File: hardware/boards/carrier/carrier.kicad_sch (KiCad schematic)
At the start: 4 parts, among them J1 XT30PW(2+2)-M.G.B_SLOT, J2 DC+_OUT, J3 DC-_OUT, J4 I2C_OUT

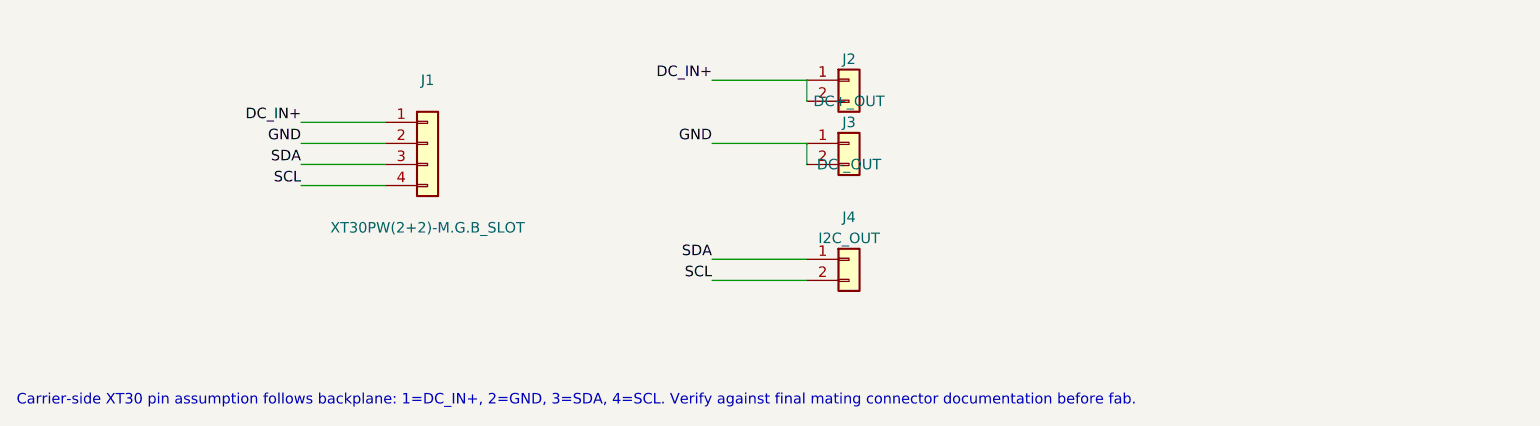
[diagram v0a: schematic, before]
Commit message: chore: checkpoint current project updates
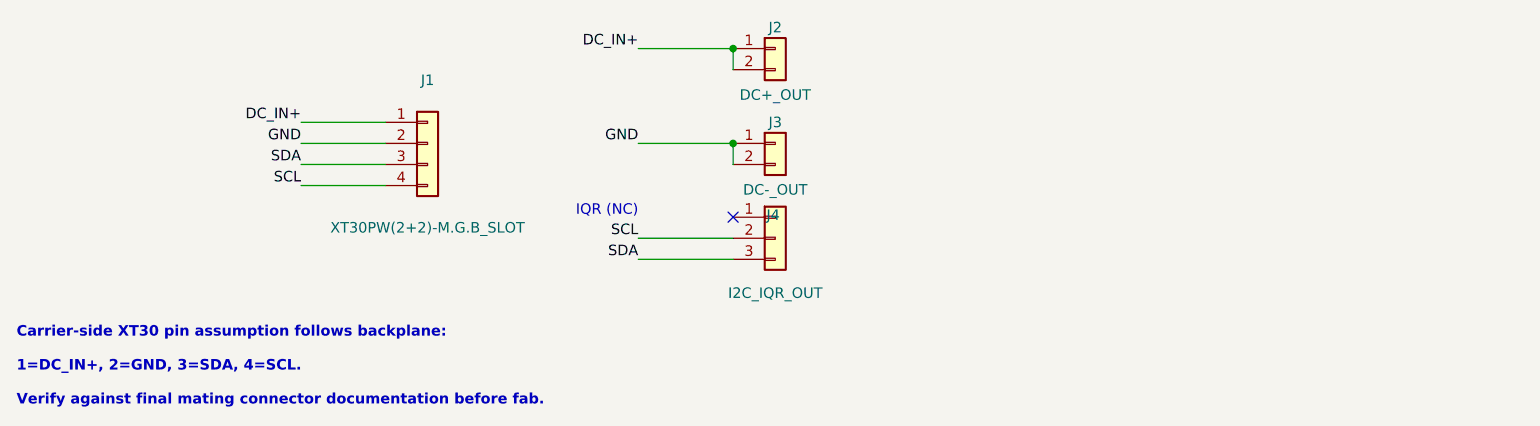
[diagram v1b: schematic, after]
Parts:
- J4: value I2C_OUT -> I2C_IQR_OUT; footprint Connector_PinHeader_2.54mm:PinHeader_1x02_P2.54mm_Vertical -> Connector_PinHeader_2.54mm:PinHeader_1x03_P2.54mm_Vertical; symbol Connector_Generic:Conn_01x02 -> Connector_Generic:Conn_01x03
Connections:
- net SDA: now also J4.3 (Pin_3); no longer J4.1 (Pin_1)
- no-connect marks 0 -> 1
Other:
- note added: "IQR (NC)"
- moved on the sheet: J2, J3
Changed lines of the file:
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@@
 		(rev "A")
 	)
-	(text "Carrier-side XT30 pin assumption follows backplane: 1=DC_IN+, 2=GND, 3=SDA, 4=SCL. Verify against final mating connector documentation before fab."
+	(text "Carrier-side XT30 pin assumption follows backplane: \n\n1=DC_IN+, 2=GND, 3=SDA, 4=SCL. \n\nVerify against final mating connector documentation before fab."
 		(exclude_from_sim no)
 		(at 35.56 82.55 0)
 		(effects
 			(font
-				(size 1.27 1.27)
+				(face "JetBrainsMono NF")
+				(size 1.27 1.27)
+				(bold yes)
 			)
 			(justify left bottom)
 		)
 	)
+	(text "IQR (NC)"
+		(exclude_from_sim no)
+		(at 110.49 59.69 0)
+		(effects
+			(font
+				(size 1.27 1.27)
+			)
+			(justify right bottom)
+		)
+	)
+	(junction
+		(at 121.92 39.37)
+		(diameter 0)
+		(color 0 0 0 0)
+	)
+	(junction
+		(at 121.92 50.8)
+		(diameter 0)
+		(color 0 0 0 0)
+	)
+	(no_connect
+		(at 121.92 59.69)
+	)
 	(wire
 		(pts
@@
 	(wire
 		(pts
-			(xy 119.38 43.18) (xy 130.81 43.18)
-		)
-		(stroke
-			(width 0)
-			(type default)
-		)
-	)
-	(wire
-		(pts
-			(xy 130.81 43.18) (xy 130.81 45.72)
-		)
-		(stroke
-			(width 0)
-			(type default)
-		)
-	)
-	(wire
-		(pts
-			(xy 119.38 50.8) (xy 130.81 50.8)
-		)
-		(stroke
-			(width 0)
-			(type default)
-		)
-	)
-	(wire
-		(pts
-			(xy 130.81 50.8) (xy 130.81 53.34)
-		)
-		(stroke
-			(width 0)
-			(type default)
-		)
-	)
-	(wire
-		(pts
-			(xy 119.38 64.77) (xy 130.81 64.77)
-		)
-		(stroke
-			(width 0)
-			(type default)
-		)
-	)
-	(wire
-		(pts
-			(xy 119.38 67.31) (xy 130.81 67.31)
+			(xy 110.49 39.37) (xy 121.92 39.37)
+		)
+		(stroke
+			(width 0)
+			(type default)
+		)
+	)
+	(wire
+		(pts
+			(xy 110.49 50.8) (xy 121.92 50.8)
+		)
+		(stroke
+			(width 0)
+			(type default)
+		)
+	)
+	(wire
+		(pts
+			(xy 110.49 62.23) (xy 121.92 62.23)
+		)
+		(stroke
+			(width 0)
+			(type default)
+		)
+	)
+	(wire
+		(pts
+			(xy 110.49 64.77) (xy 121.92 64.77)
+		)
+		(stroke
+			(width 0)
+			(type default)
+		)
+	)
+	(wire
+		(pts
+			(xy 121.92 39.37) (xy 121.92 41.91)
+		)
+		(stroke
+			(width 0)
+			(type default)
+		)
+	)
+	(wire
+		(pts
+			(xy 121.92 50.8) (xy 121.92 53.34)
 		)
 		(stroke
@@
 	)
 	(label "DC_IN+"
-		(at 119.38 43.18 180)
+		(at 110.49 39.37 180)
 		(effects
 			(font
@@
 	)
 	(label "GND"
-		(at 119.38 50.8 180)
+		(at 110.49 50.8 180)
+		(effects
+			(font
+				(size 1.27 1.27)
+			)
+			(justify right bottom)
+		)
+	)
+	(label "SCL"
+		(at 110.49 62.23 180)
 		(effects
 			(font
@@
 	)
 	(label "SDA"
-		(at 119.38 64.77 180)
-		(effects
-			(font
-				(size 1.27 1.27)
-			)
-			(justify right bottom)
-		)
-	)
-	(label "SCL"
-		(at 119.38 67.31 180)
+		(at 110.49 64.77 180)
 		(effects
 			(font
@@
 	(symbol
 		(lib_id "Connector_Generic:Conn_01x02")
-		(at 135.89 43.18 0)
+		(at 127 39.37 0)
 		(unit 1)
 		(body_style 1)
@@
 		(dnp no)
 		(property "Reference" "J2"
-			(at 135.89 40.64 0)
+			(at 127 36.83 0)
 			(show_name no)
 			(do_not_autoplace no)
@@
 		)
 		(property "Value" "DC+_OUT"
-			(at 135.89 45.72 0)
+			(at 127 44.958 0)
 			(show_name no)
 			(do_not_autoplace no)
@@
 		)
 		(property "Footprint" "Connector_PinHeader_2.54mm:PinHeader_1x02_P2.54mm_Vertical"
-			(at 135.89 43.18 0)
+			(at 127 39.37 0)
 			(hide yes)
 			(show_name no)
@@
 		)
 		(property "Datasheet" ""
-			(at 135.89 43.18 0)
+			(at 127 39.37 0)
 			(hide yes)
 			(show_name no)
@@
 		)
 		(property "Description" "Two-pin breakout for carrier DC input positive"
-			(at 135.89 43.18 0)
+			(at 127 39.37 0)
 			(hide yes)
 			(show_name no)
@@
 	(symbol
 		(lib_id "Connector_Generic:Conn_01x02")
-		(at 135.89 50.8 0)
+		(at 127 50.8 0)
 		(unit 1)
 		(body_style 1)
@@
 		(dnp no)
 		(property "Reference" "J3"
-			(at 135.89 48.26 0)
+			(at 127 48.26 0)
 			(show_name no)
 			(do_not_autoplace no)
@@
 		)
 		(property "Value" "DC-_OUT"
-			(at 135.89 53.34 0)
+			(at 127 56.388 0)
 			(show_name no)
 			(do_not_autoplace no)
@@
 		)
 		(property "Footprint" "Connector_PinHeader_2.54mm:PinHeader_1x02_P2.54mm_Vertical"
-			(at 135.89 50.8 0)
+			(at 127 50.8 0)
 			(hide yes)
 			(show_name no)
@@
 		)
 		(property "Datasheet" ""
-			(at 135.89 50.8 0)
+			(at 127 50.8 0)
 			(hide yes)
 			(show_name no)
@@
 		)
 		(property "Description" "Two-pin breakout for carrier DC input return"
-			(at 135.89 50.8 0)
+			(at 127 50.8 0)
 			(hide yes)
 			(show_name no)
@@
 	)
 	(symbol
-		(lib_id "Connector_Generic:Conn_01x02")
-		(at 135.89 64.77 0)
+		(lib_id "Connector_Generic:Conn_01x03")
+		(at 127 62.23 0)
 		(unit 1)
 		(body_style 1)
@@
 		(dnp no)
 		(property "Reference" "J4"
-			(at 135.89 59.69 0)
-			(show_name no)
-			(do_not_autoplace no)
-			(effects
-				(font
-					(size 1.27 1.27)
-				)
-			)
-		)
-		(property "Value" "I2C_OUT"
-			(at 135.89 62.23 0)
-			(show_name no)
-			(do_not_autoplace no)
-			(effects
-				(font
-					(size 1.27 1.27)
-				)
-			)
-		)
-		(property "Footprint" "Connector_PinHeader_2.54mm:PinHeader_1x02_P2.54mm_Vertical"
-			(at 135.89 64.77 0)
+			(at 126.746 59.436 0)
+			(show_name no)
+			(do_not_autoplace no)
+			(effects
+				(font
+					(size 1.27 1.27)
+				)
+			)
+		)
+		(property "Value" "I2C_IQR_OUT"
+			(at 127 68.834 0)
+			(show_name no)
+			(do_not_autoplace no)
+			(effects
+				(font
+					(size 1.27 1.27)
+				)
+			)
+		)
+		(property "Footprint" "Connector_PinHeader_2.54mm:PinHeader_1x03_P2.54mm_Vertical"
+			(at 127 62.23 0)
 			(hide yes)
 			(show_name no)
@@
 		)
 		(property "Datasheet" ""
-			(at 135.89 64.77 0)
-			(hide yes)
-			(show_name no)
-			(do_not_autoplace no)
-			(effects
-				(font
-					(size 1.27 1.27)
-				)
-			)
-		)
-		(property "Description" "Two-pin breakout for carrier I2C bus"
-			(at 135.89 64.77 0)
+			(at 127 62.23 0)
+			(hide yes)
+			(show_name no)
+			(do_not_autoplace no)
+			(effects
+				(font
+					(size 1.27 1.27)
+				)
+			)
+		)
+		(property "Description" "Three-pin breakout for carrier I2C bus with reserved IQR"
+			(at 127 62.23 0)
 			(hide yes)
 			(show_name no)
@@
 		(pin "2"
 		)
+		(pin "3"
+		)
 		(instances
